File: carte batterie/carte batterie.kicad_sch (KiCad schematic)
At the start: 29 parts, among them IC1 TPS3711DDCT, IC2 TPS54531DDA, J1 Conn_01x02_Pin, J2 Conn_01x02_Pin, J3 Conn_01x01_Pin, J4 Conn_01x02_Pin, Q1 SI3127DV-T1-GE3, U1 ATtiny1616-S

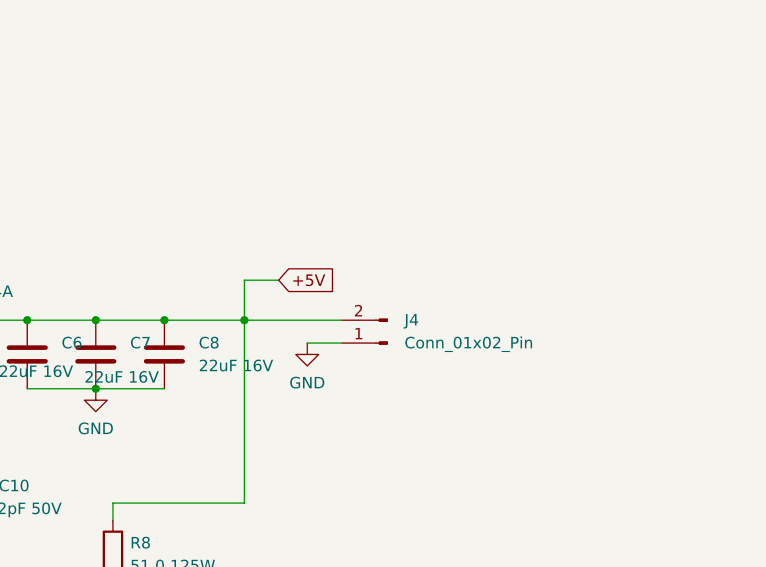
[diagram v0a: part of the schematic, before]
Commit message: modif
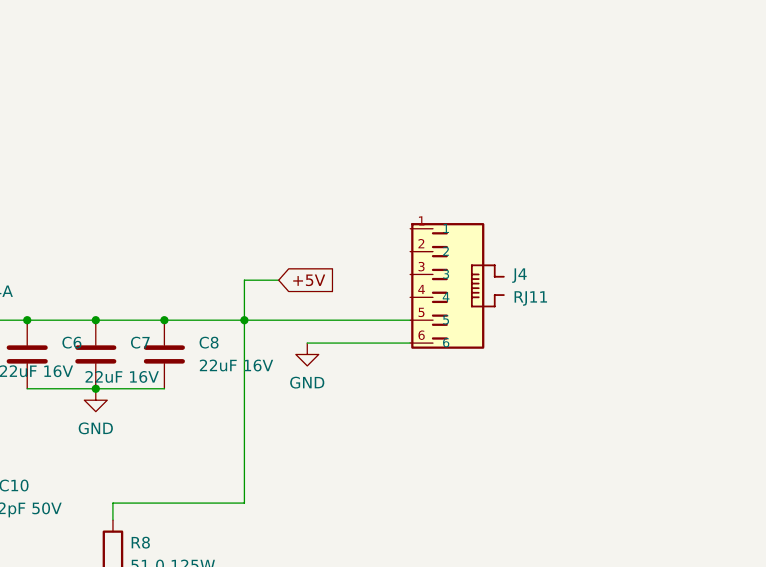
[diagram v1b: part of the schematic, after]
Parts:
- removed J4: Conn_01x02_Pin, symbol Connector:Conn_01x02_Pin
- added J4: RJ11, symbol RJ11:RJ11
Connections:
- net +5V: now also J4.5
- net GND: now also J4.6
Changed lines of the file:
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@@
     (stroke (width 0) (type default))
   )
-  (wire (pts (xy 193.675 118.745) (xy 197.485 118.745))
+  (wire (pts (xy 193.675 118.745) (xy 205.105 118.745))
     (stroke (width 0) (type default))
   )
@@
     (stroke (width 0) (type default))
   )
-  (wire (pts (xy 186.69 116.205) (xy 197.485 116.205))
+  (wire (pts (xy 186.69 116.205) (xy 205.105 116.205))
     (stroke (width 0) (type default))
   )
@@
     )
   )
-  (symbol (lib_id "Connector:Conn_01x02_Pin") (at 202.565 118.745 180) (unit 1)
-    (in_bom yes) (on_board yes) (dnp no) (fields_autoplaced)
-    (property "Reference" "J4" (at 204.47 116.205 0)
-      (effects (font (size 1.27 1.27)) (justify right))
-    )
-    (property "Value" "Conn_01x02_Pin" (at 204.47 118.745 0)
-      (effects (font (size 1.27 1.27)) (justify right))
-    )
-    (property "Footprint" "" (at 202.565 118.745 0)
-      (effects (font (size 1.27 1.27)) hide)
-    )
-    (property "Datasheet" "~" (at 202.565 118.745 0)
-      (effects (font (size 1.27 1.27)) hide)
+  (symbol (lib_id "RJ11:RJ11") (at 207.645 111.125 0) (unit 1)
+    (in_bom yes) (on_board yes) (dnp no) (fields_autoplaced)
+    (property "Reference" "J4" (at 216.535 111.125 0)
+      (effects (font (size 1.27 1.27)) (justify left))
+    )
+    (property "Value" "RJ11" (at 216.535 113.665 0)
+      (effects (font (size 1.27 1.27)) (justify left))
+    )
+    (property "Footprint" "" (at 207.645 111.125 0)
+      (effects (font (size 1.27 1.27)) hide)
+    )
+    (property "Datasheet" "" (at 207.645 111.125 0)
+      (effects (font (size 1.27 1.27)) hide)
+    )
+    (property "MF" "" (at 207.645 111.125 0)
+      (effects (font (size 1.27 1.27)) (justify bottom) hide)
+    )
+    (property "Description" "\n" (at 207.645 111.125 0)
+      (effects (font (size 1.27 1.27)) (justify bottom) hide)
+    )
+    (property "Package" "" (at 207.645 111.125 0)
+      (effects (font (size 1.27 1.27)) (justify bottom) hide)
+    )
+    (property "Price" "" (at 207.645 111.125 0)
+      (effects (font (size 1.27 1.27)) (justify bottom) hide)
+    )
+    (property "SnapEDA_Link" "" (at 207.645 111.125 0)
+      (effects (font (size 1.27 1.27)) (justify bottom) hide)
+    )
+    (property "MP" "" (at 207.645 111.125 0)
+      (effects (font (size 1.27 1.27)) (justify bottom) hide)
+    )
+    (property "Availability" "" (at 207.645 111.125 0)
+      (effects (font (size 1.27 1.27)) (justify bottom) hide)
+    )
+    (property "Check_prices" "" (at 207.645 111.125 0)
+      (effects (font (size 1.27 1.27)) (justify bottom) hide)
     )
     (pin "1")
     (pin "2")
-    (instances
-      (project "carte batterie"
+    (pin "3")
+    (pin "4")
+    (pin "5")
+    (pin "6")
+    (instances
+      (project "carte batterie"

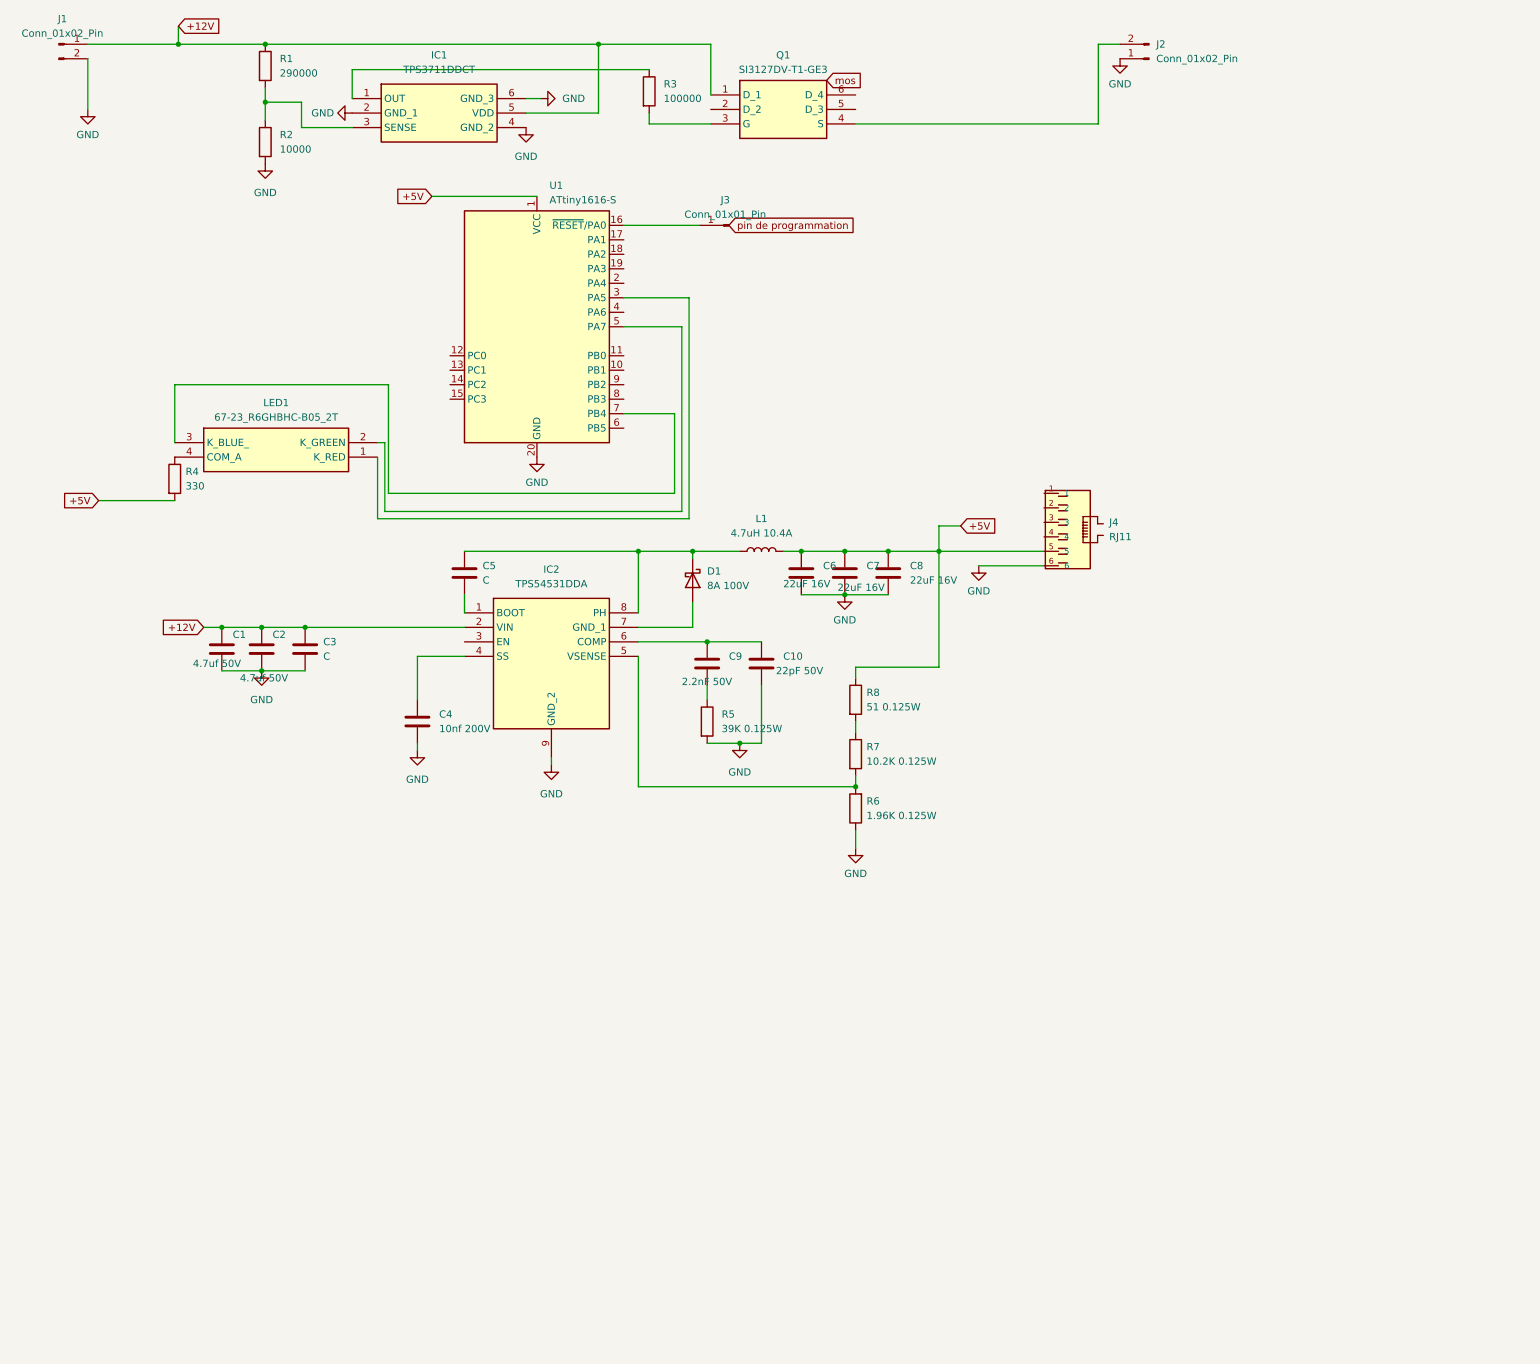
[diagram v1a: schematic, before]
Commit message: carte bat
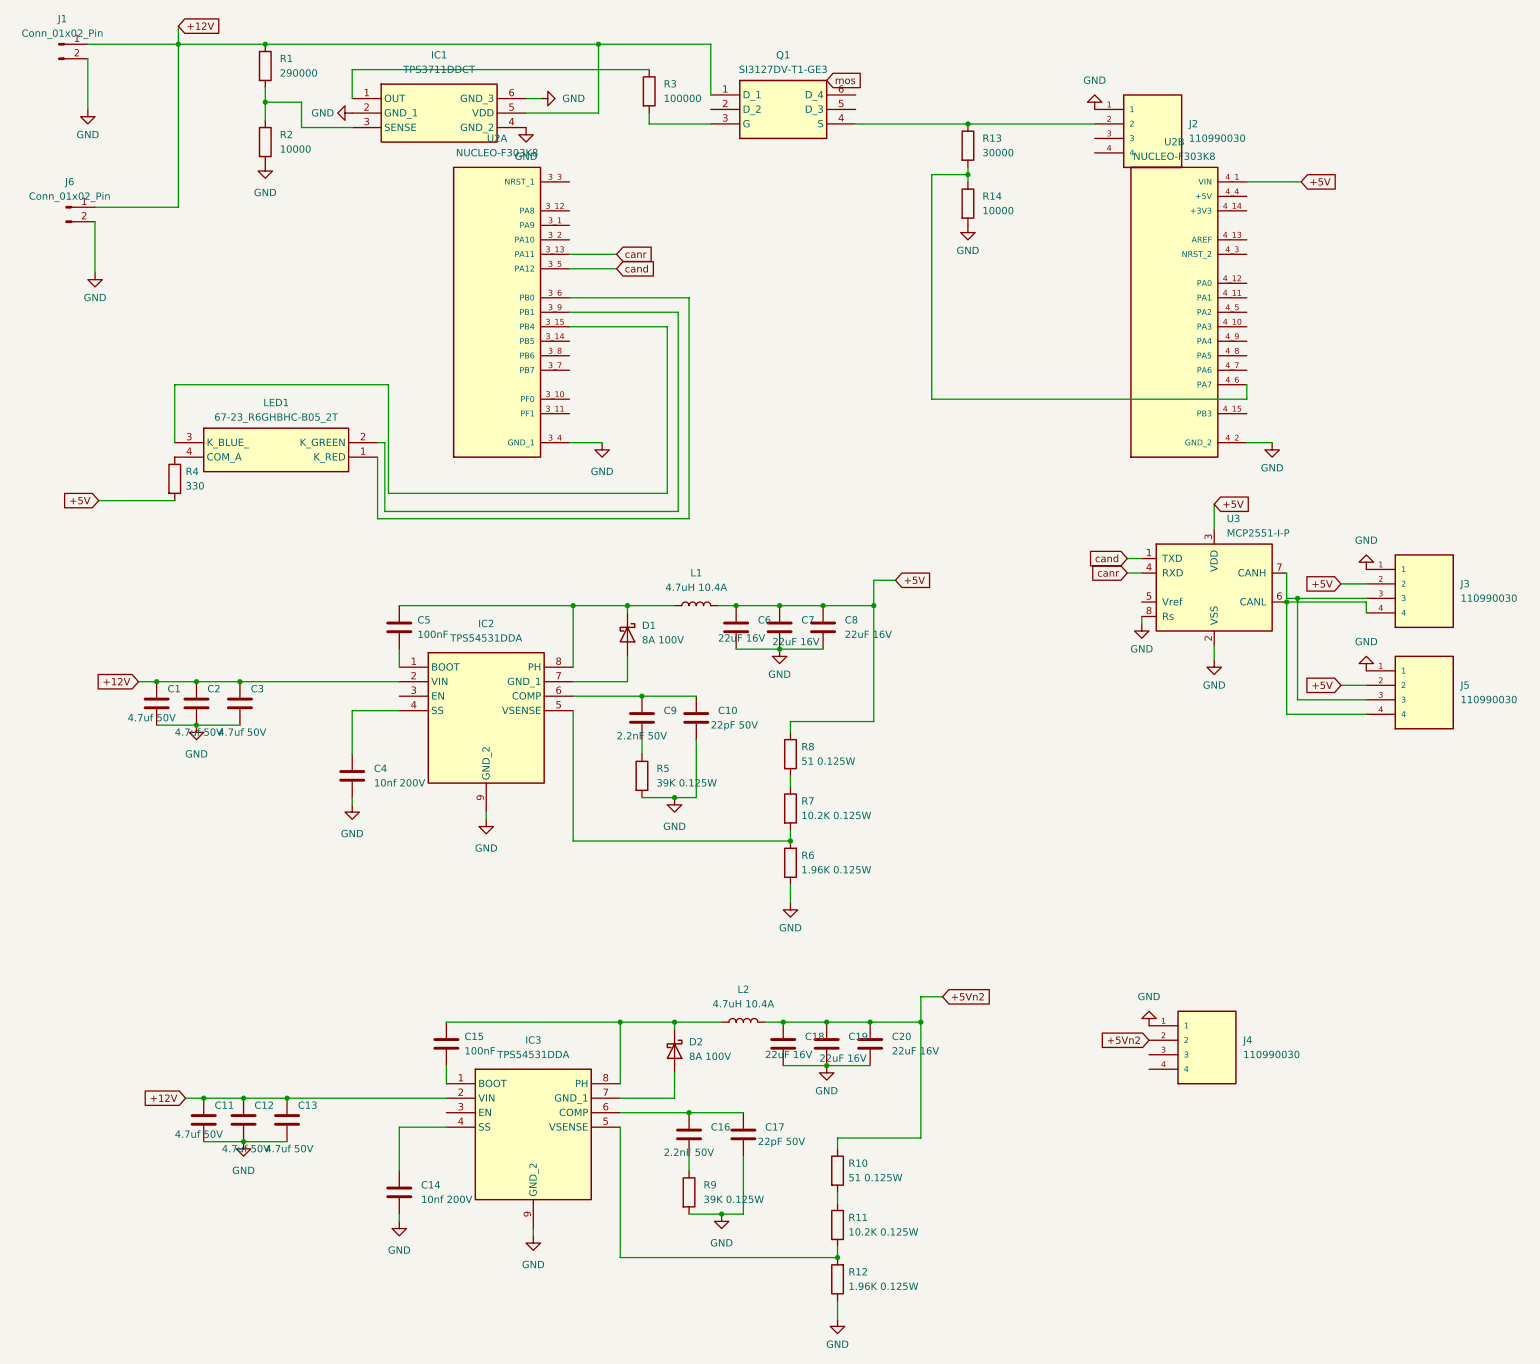
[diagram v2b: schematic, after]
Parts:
- removed J2: Conn_01x02_Pin, symbol Connector:Conn_01x02_Pin
- removed J3: Conn_01x01_Pin, symbol Connector:Conn_01x01_Pin
- removed J4: RJ11, symbol RJ11:RJ11
- removed U1: ATtiny1616-S, Package_SO:SOIC-20W_7.5x12.8mm_P1.27mm, symbol MCU_Microchip_ATtiny:ATtiny1616-S
- added C11, C12, C13: 4.7uf 50V, Capacitor_SMD:C_0805_2012Metric, symbol Device:C
- added C14: 10nf 200V, Capacitor_SMD:C_0805_2012Metric, symbol Device:C
- added C15: 100nF, symbol Device:C
- added C16: 2.2nF 50V, Capacitor_SMD:C_0603_1608Metric, symbol Device:C
- added C17: 22pF 50V, Capacitor_SMD:C_0805_2012Metric, symbol Device:C
- added C18, C19, C20: 22uF 16V, Capacitor_SMD:C_0805_2012Metric, symbol Device:C
- added D2: 8A 100V, Package_TO_SOT_SMD:TO-277A, symbol Device:D_Schottky
- added IC3: TPS54531DDA, SOIC127P600X170-9N, symbol SamacSys_Parts:TPS54531DDA
- added J2, J3, J4, J5: 110990030, symbol 110990030:110990030
- added J6: Conn_01x02_Pin, symbol Connector:Conn_01x02_Pin
- added L2: 4.7uH 10.4A, Inductor_SMD:L_Wuerth_HCI-1040, symbol Device:L
- added R10: 51 0.125W, Resistor_SMD:R_0805_2012Metric, symbol Device:R
- added R11: 10.2K 0.125W, Capacitor_SMD:C_0805_2012Metric, symbol Device:R
- added R12: 1.96K 0.125W, Capacitor_SMD:C_0805_2012Metric, symbol Device:R
- added R13: 30000, symbol Device:R
- added R14: 10000, symbol Device:R
- added R9: 39K 0.125W, Capacitor_SMD:C_0805_2012Metric, symbol Device:R
- added U2: NUCLEO-F303K8, symbol NUCLEO-F303K8:NUCLEO-F303K8
- added U3: MCP2551-I-P, Package_DIP:DIP-8_W7.62mm, symbol Interface_CAN_LIN:MCP2551-I-P
- C3: value C -> 4.7uf 50V; footprint (none) -> Capacitor_SMD:C_0805_2012Metric
- C5: value C -> 100nF
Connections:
- net +12V: now also C11.1, C12.1, C13.1, IC3.2 (VIN), J6.1 (Pin_1)
- net +5V: now also J3.2, J5.2, U2.4_1 (VIN), U3.3 (VDD)
- net GND: now also C11.2, C12.2, C13.2, C14.2, C17.2, C18.2, C19.2, C20.2, IC3.9 (GND_2), J2.1, J3.1, J4.1, J5.1, J6.2 (Pin_2), R12.1, R14.2, R9.2, U2.3_4 (GND_1), U2.4_2 (GND_2), U3.2 (VSS), U3.8 (Rs)
- net at LED1.1 (K_RED): now also U2.3_6 (PB0)
- net at LED1.2 (K_GREEN): now also U2.3_9 (PB1)
- net at LED1.3 (K_BLUE_): now also U2.3_15 (PB4)
- net at Q1.4 (S): now also J2.2, R13.1
- new net: R13.2, R14.1, U2.4_6 (PA7)
- new net: C16.1, C17.1, IC3.6 (COMP)
- new net: C16.2, R9.1
- new net: C15.2, IC3.1 (BOOT)
- new net: C14.1, IC3.4 (SS)
- new net: IC3.5 (VSENSE), R11.2, R12.2
- new net: D2.2 (A), IC3.7 (GND_1)
- new net: C15.1, D2.1 (K), IC3.8 (PH), L2.1
- new net: J3.4, J5.4, U3.6 (CANL)
- new net: J3.3, J5.3, U3.7 (CANH)
- new net: R10.2, R11.1
- new net +5Vn2: C18.1, C19.1, C20.1, J4.2, L2.2, R10.1
- new net cand: U2.3_5 (PA12), U3.1 (TXD)
- new net canr: U2.3_13 (PA11), U3.4 (RXD)
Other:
- moved on the sheet: C1, C10, C2, C4, C5, C6, C7, C8, C9, D1, IC2, L1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

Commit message: carte bat
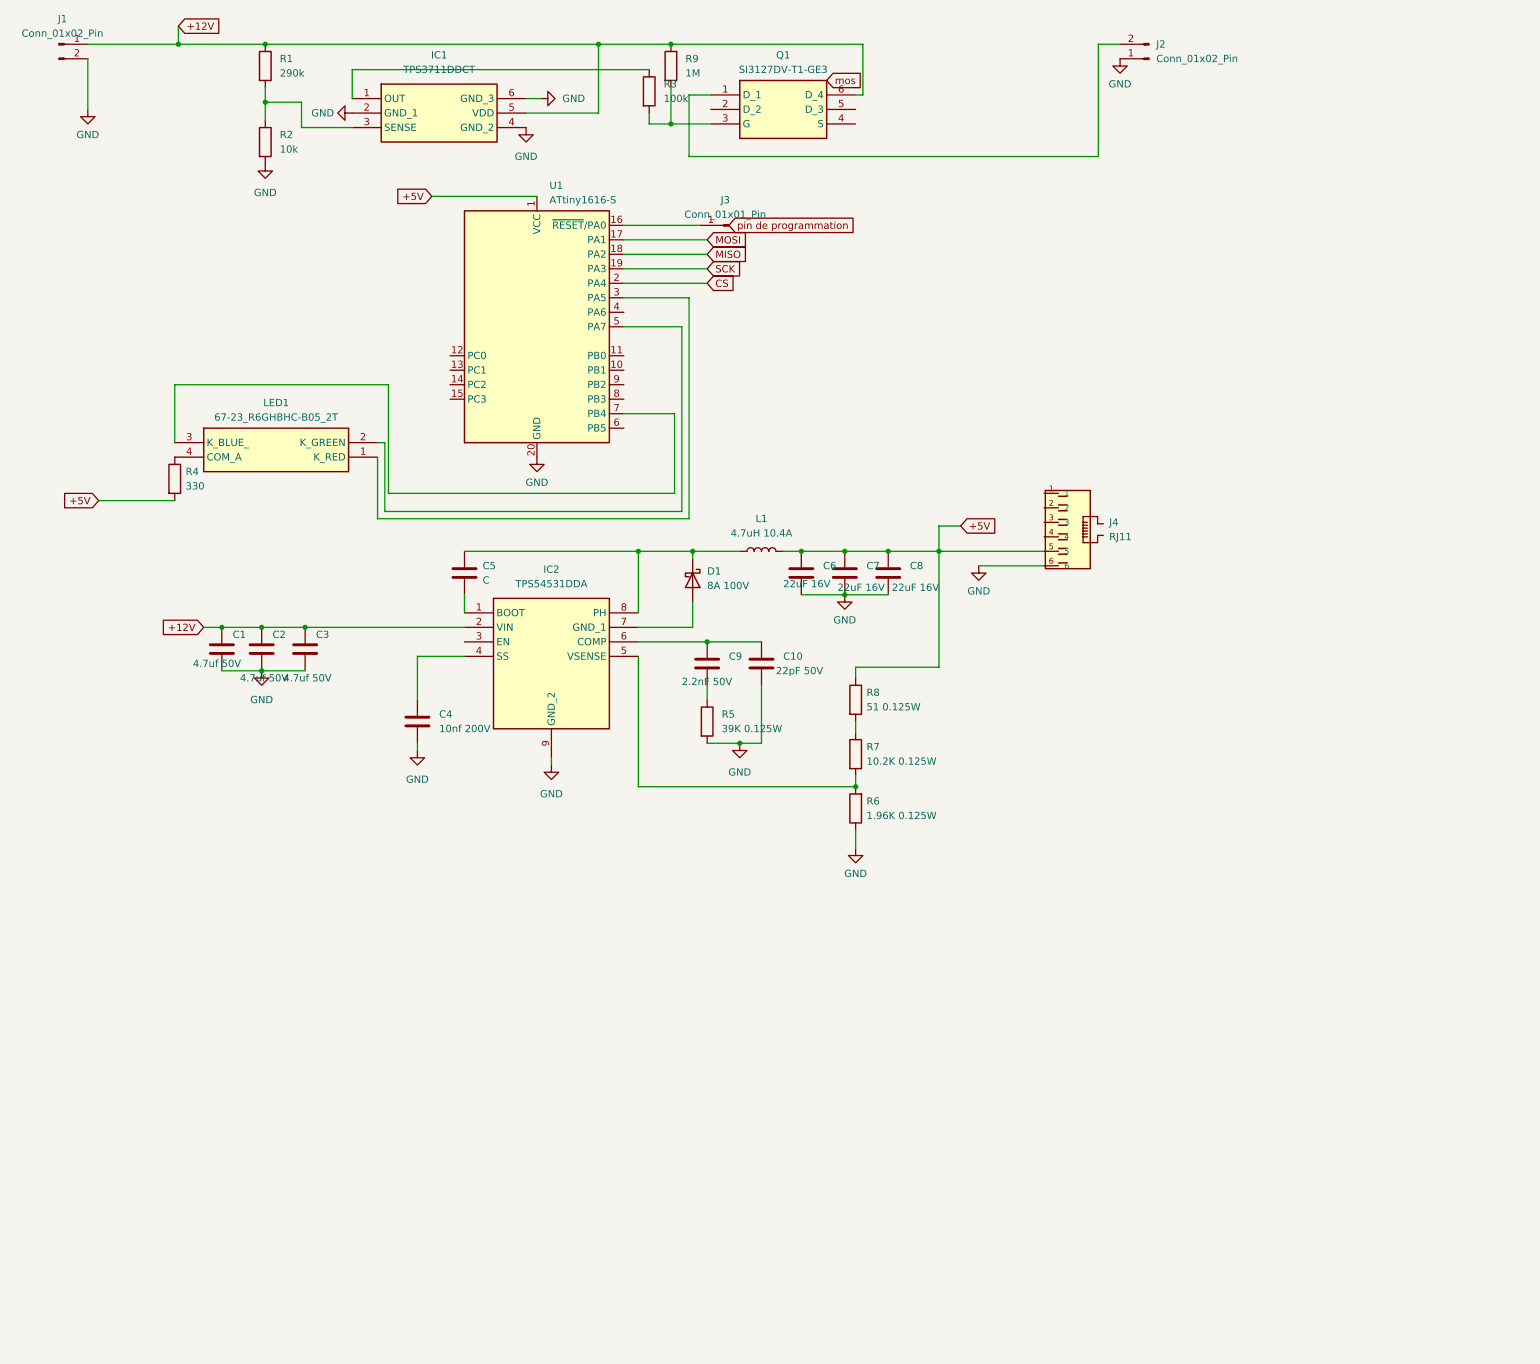
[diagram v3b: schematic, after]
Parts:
- removed C11, C12, C13: 4.7uf 50V, Capacitor_SMD:C_0805_2012Metric, symbol Device:C
- removed C14: 10nf 200V, Capacitor_SMD:C_0805_2012Metric, symbol Device:C
- removed C15: 100nF, symbol Device:C
- removed C16: 2.2nF 50V, Capacitor_SMD:C_0603_1608Metric, symbol Device:C
- removed C17: 22pF 50V, Capacitor_SMD:C_0805_2012Metric, symbol Device:C
- removed C18, C19, C20: 22uF 16V, Capacitor_SMD:C_0805_2012Metric, symbol Device:C
- removed D2: 8A 100V, Package_TO_SOT_SMD:TO-277A, symbol Device:D_Schottky
- removed IC3: TPS54531DDA, SOIC127P600X170-9N, symbol SamacSys_Parts:TPS54531DDA
- removed J2, J3, J4, J5: 110990030, symbol 110990030:110990030
- removed J6: Conn_01x02_Pin, symbol Connector:Conn_01x02_Pin
- removed L2: 4.7uH 10.4A, Inductor_SMD:L_Wuerth_HCI-1040, symbol Device:L
- removed R10: 51 0.125W, Resistor_SMD:R_0805_2012Metric, symbol Device:R
- removed R11: 10.2K 0.125W, Capacitor_SMD:C_0805_2012Metric, symbol Device:R
- removed R12: 1.96K 0.125W, Capacitor_SMD:C_0805_2012Metric, symbol Device:R
- removed R13: 30000, symbol Device:R
- removed R14: 10000, symbol Device:R
- removed U2: NUCLEO-F303K8, symbol NUCLEO-F303K8:NUCLEO-F303K8
- removed U3: MCP2551-I-P, Package_DIP:DIP-8_W7.62mm, symbol Interface_CAN_LIN:MCP2551-I-P
- added J2: Conn_01x02_Pin, symbol Connector:Conn_01x02_Pin
- added J3: Conn_01x01_Pin, symbol Connector:Conn_01x01_Pin
- added J4: RJ11, symbol RJ11:RJ11
- added U1: ATtiny1616-S, Package_SO:SOIC-20W_7.5x12.8mm_P1.27mm, symbol MCU_Microchip_ATtiny:ATtiny1616-S
- C5: value 100nF -> C
- R1: value 290000 -> 290k
- R2: value 10000 -> 10k
- R3: value 100000 -> 100k
- R9: value 39K 0.125W -> 1M; footprint Capacitor_SMD:C_0805_2012Metric -> (none)
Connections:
- net +12V: now also Q1.6 (D_4), R9.1; no longer Q1.1 (D_1)
- net +5V: now also J4.5, U1.1 (VCC)
- net GND: now also J2.1 (Pin_1), J4.6, U1.20 (GND); no longer R9.2
- net at Q1.3 (G), R3.2: now also R9.2
- net at LED1.1 (K_RED): now also U1.3 (PA5)
- net at LED1.2 (K_GREEN): now also U1.5 (PA7)
- net at LED1.3 (K_BLUE_): now also U1.7 (PB4)
- new net: J3.1 (Pin_1), U1.16 (~{RESET}/PA0)
- new net: J2.2 (Pin_2), Q1.1 (D_1)
- new net CS: U1.2 (PA4)
- new net MISO: U1.18 (PA2)
- new net MOSI: U1.17 (PA1)
- new net SCK: U1.19 (PA3)
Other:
- moved on the sheet: C1, C10, C2, C4, C5, C6, C7, C8, C9, D1, IC2, L1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
